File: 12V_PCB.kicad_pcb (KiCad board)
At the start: 2 copper layers, 21.5 x 37.5 mm, 13 parts, among them J1 12V IN, J11 LED_STRIP, J2 RPI CONN, J21 LED_BTN, J3 BTN, Q11 PMV40UN2R, Q21 PMV40UN2R

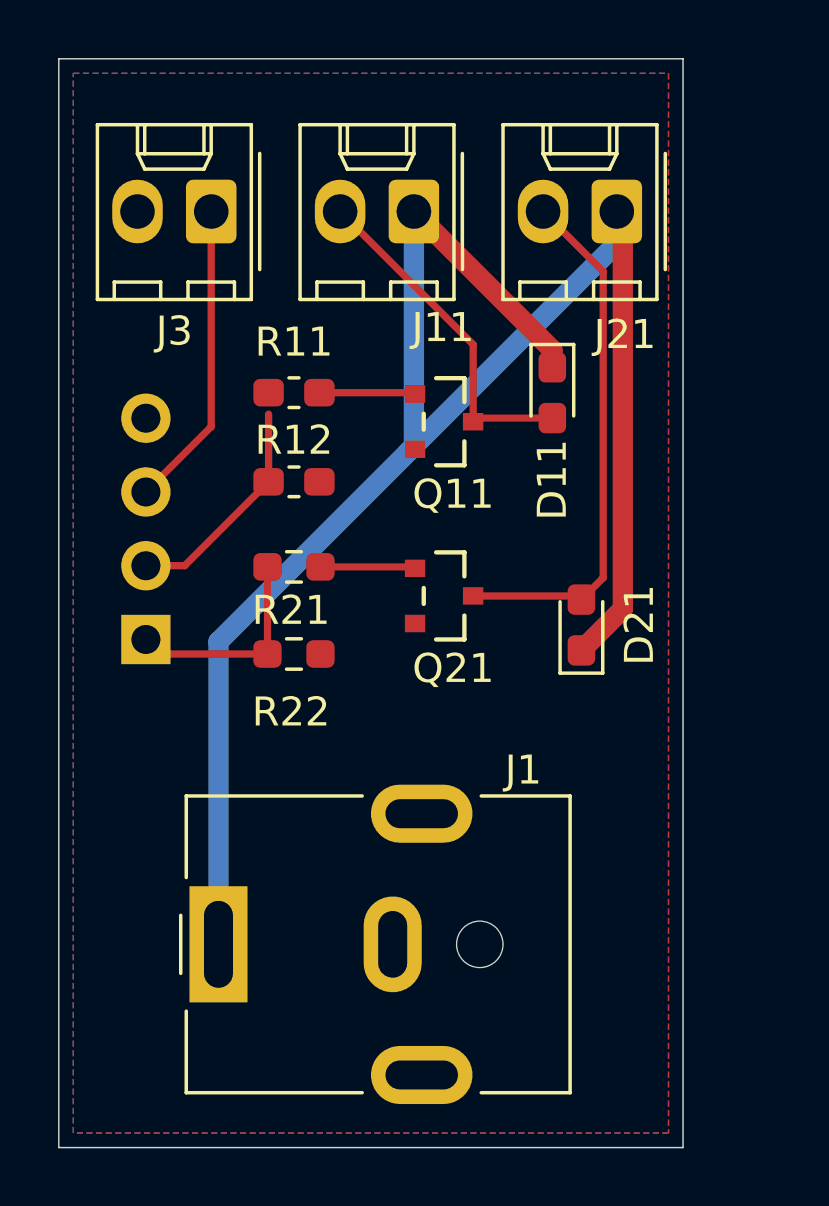
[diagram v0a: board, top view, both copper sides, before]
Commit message: Final version with panelization
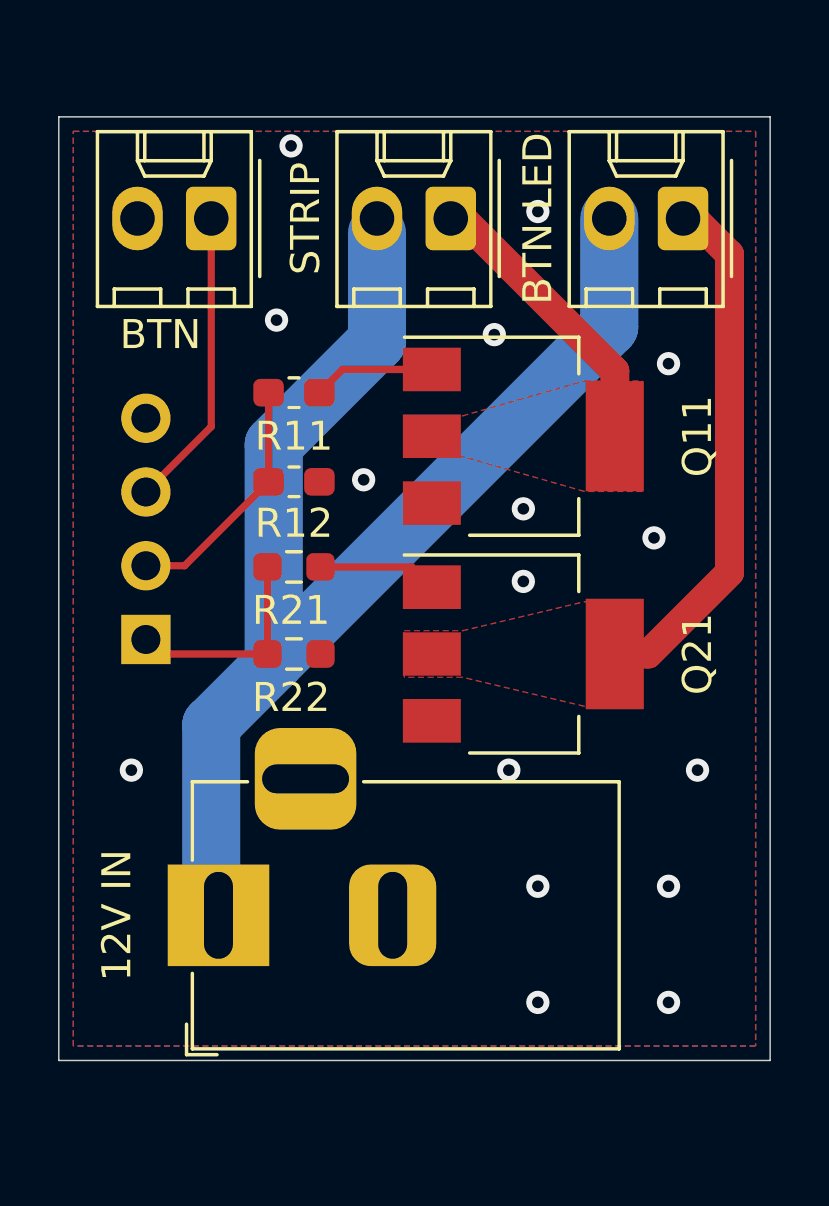
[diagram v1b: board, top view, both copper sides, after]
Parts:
- removed D11, D21: SL04-E3-08, Diode_SMD:D_0603_1608Metric_Pad1.05x0.95mm_HandSolder
- J1: footprint Connector_BarrelJack:BarrelJack_CUI_PJ-063AH_Horizontal -> Connector_BarrelJack:BarrelJack_Horizontal
- Q11, Q21: value PMV40UN2R -> IRLL2705PBF; footprint PMV40UN2R:Nexperia-SOT23-01_2018-0-0 -> Package_TO_SOT_SMD:SOT-223-3_TabPin2
- moved Q21 3.38 mm to (169.5, 127.0), turned to 0 degrees
- moved Q11 2.78 mm to (169.5, 119.5), turned to 0 degrees
- moved J21 2.29 mm to (175.0, 112.0)
- moved J11 1.29 mm to (167.0, 112.0)
- moved J1 1.00 mm to (159.0, 136.0), turned to 180 degrees
- moved J3 0.24 mm to (158.8, 112.0)
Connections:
- J11 pad 1: +12V -> Net-(J11-Pad1)
- J11 pad 2: Net-(D11-Pad2) -> +12V
- J21 pad 1: +12V -> Net-(J21-Pad1)
- J21 pad 2: Net-(D21-Pad2) -> +12V
- Q11 pad 2: GND -> Net-(J11-Pad1)
- Q11 pad 3: Net-(D11-Pad2) -> GND
- Q21 pad 2: GND -> Net-(J21-Pad1)
- Q21 pad 3: Net-(D21-Pad2) -> GND
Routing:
- net Net-(D21-Pad2): track 18.3 -> 0.00 mm
- net Net-(J21-Pad1): track 0.00 -> 18.2 mm
- net +12V: track 63.0 -> 46.0 mm
- net Net-(D11-Pad2): track 11.9 -> 0.00 mm
- net Net-(J11-Pad1): track 0.00 -> 10.1 mm
- net Net-(Q11-Pad1): track 3.32 -> 4.21 mm
- net Net-(Q21-Pad1): track 3.28 -> 4.13 mm
- net LED_STRIP: track 7.75 -> 8.49 mm
- net GND: vias 0 -> 16
- added copper zone on F.Cu, net Net-(J11-Pad1)
- added copper zone on F.Cu, net Net-(J21-Pad1)
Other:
- board size 21.5 x 37.5 mm -> 24.5 x 32.5 mm
- net class +12V: clearance 0.2 -> 0.5; trace_width 0.7 -> 2
- net class 12V signal added: clearance 0.2, trace_width 1, via_dia 0.8, via_drill 0.4
- board text added: "+12V"
- board text added: "12V IN"
- board text added: "BTN"
- board text added: "BTN LED"
- board text added: "GND"
- board text added: "LED_BTN"
- board text added: "STRIP"
